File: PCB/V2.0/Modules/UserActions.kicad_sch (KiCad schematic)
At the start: 12 parts, among them SW1 SW_Left, SW2 SW_Up, SW3 SW_Right, SW4 SW_Down, SW6 RotaryEncoder_Switch, SW7 SW_Center

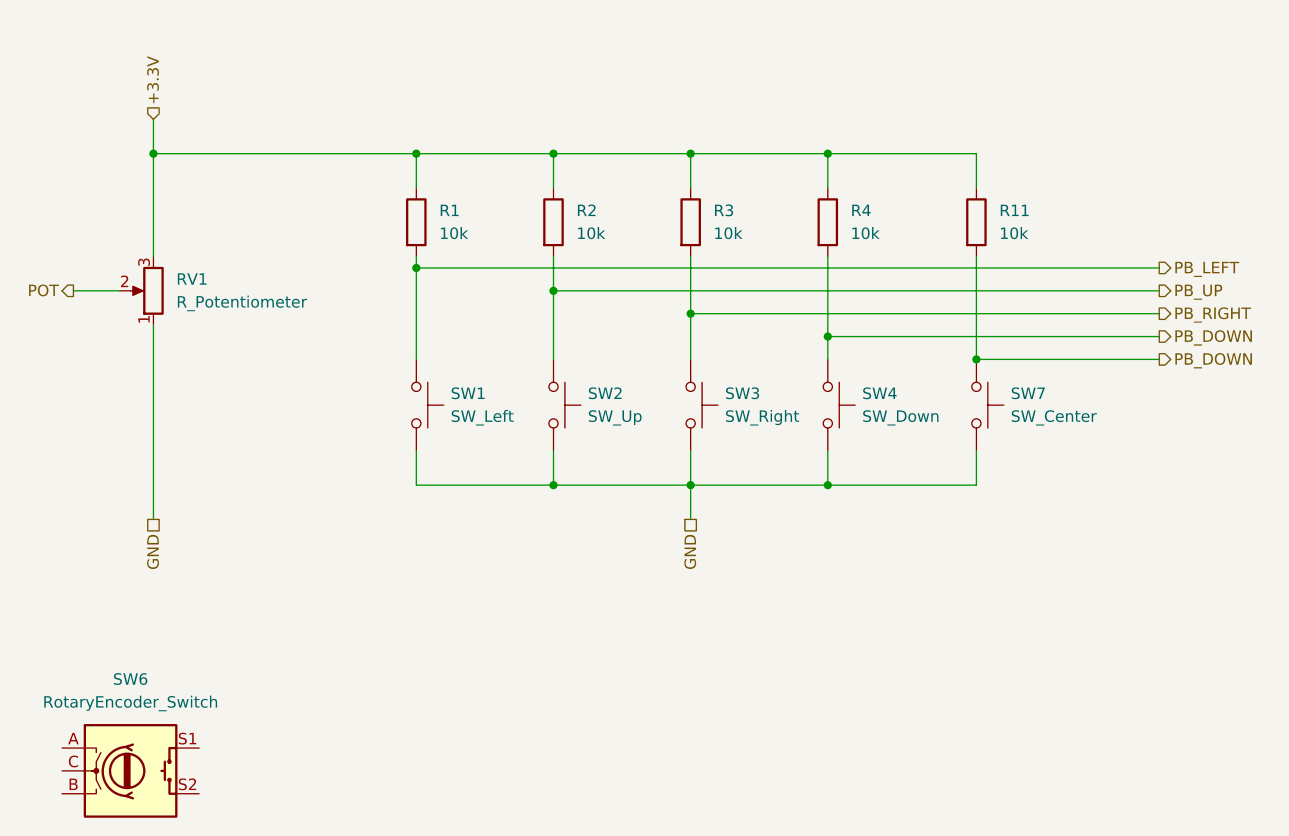
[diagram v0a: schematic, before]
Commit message: Add RTC
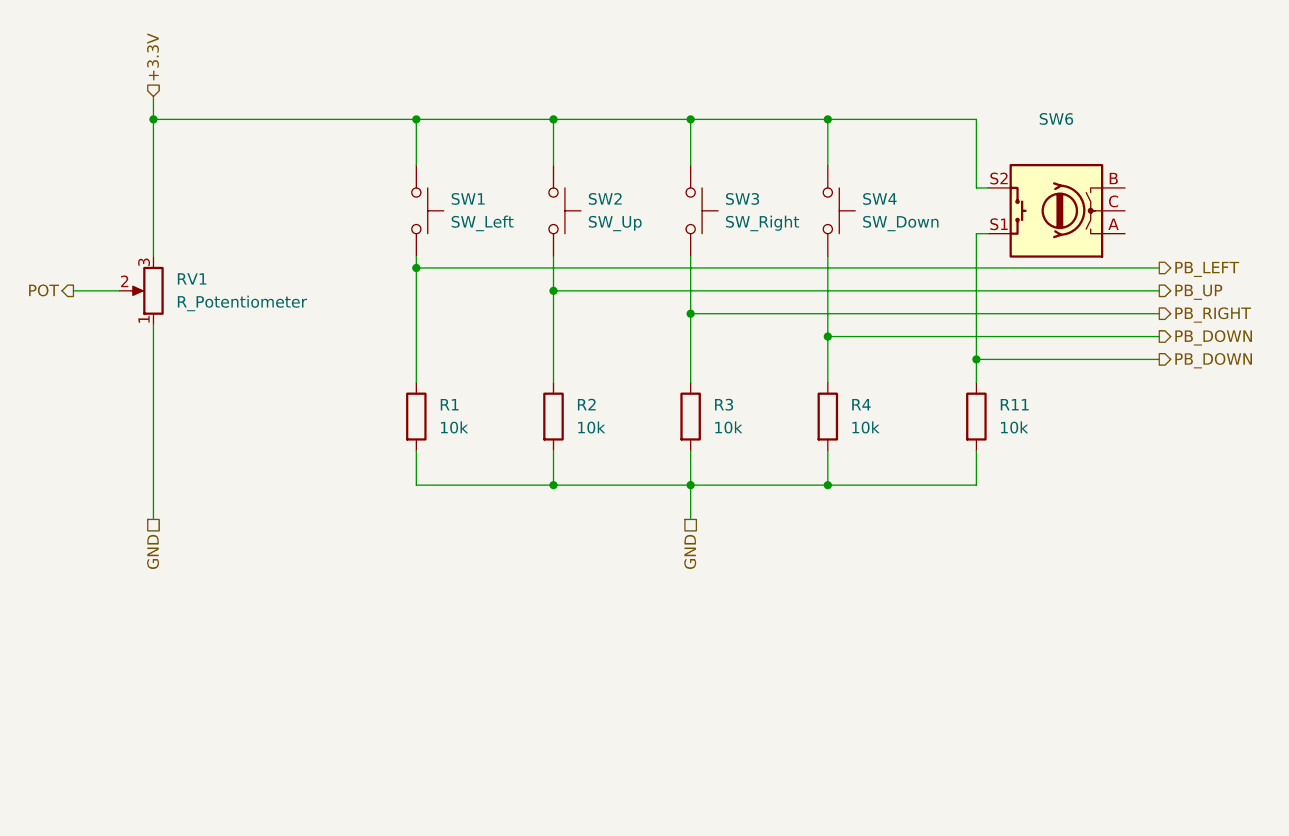
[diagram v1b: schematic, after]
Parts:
- removed SW7: SW_Center, Button_Switch_THT:SW_PUSH_6mm, symbol Switch:SW_Push
- R1, R11, R2, R3, R4: footprint Resistor_THT:R_Axial_DIN0207_L6.3mm_D2.5mm_P7.62mm_Horizontal -> Resistor_THT:R_Axial_DIN0207_L6.3mm_D2.5mm_P10.16mm_Horizontal
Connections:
- net +3.3V: now also SW1.1, SW2.1, SW3.1, SW4.1, SW6.S2; no longer R1.1, R11.1, R2.1, R3.1, R4.1
- net GND: now also R1.2, R11.2, R2.2, R3.2, R4.2; no longer SW1.2, SW2.2, SW3.2, SW4.2
- net PB_DOWN: now also R11.1, R4.1, SW4.2, SW6.S1; no longer R11.2, R4.2, SW4.1
- net PB_LEFT: now also R1.1, SW1.2; no longer R1.2, SW1.1
- net PB_RIGHT: now also R3.1, SW3.2; no longer R3.2, SW3.1
- net PB_UP: now also R2.1, SW2.2; no longer R2.2, SW2.1
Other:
- moved on the sheet: R1, R2, R3, R4, SW1, SW2, SW3, SW4, SW6
